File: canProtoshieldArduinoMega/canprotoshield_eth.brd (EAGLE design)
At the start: 101.3 x 80.6 mm, 54 parts, among them CN1 1X4-3.5MM, CN12 1X4-3.5MM, CN13 1X4-3.5MM, CN14 1X4-3.5MM, CN15 1X4-3.5MM, CN16 1X4-3.5MM, CN17 1X4-3.5MM, CN18 1X4-3.5MM, CN19 1X4-3.5MM, CN2 1X4-3.5MM, CN20 1X4-3.5MM, CN21 1X4-3.5MM, CN22 1X4-3.5MM, CN23 1X4-3.5MM, CN24 1X4-3.5MM, CN25 1X4-3.5MM, CN27 1X4-3.5MM, CN28 1X4-3.5MM, CN29 1X4-3.5MM, CN3 1X4-3.5MM, CN33 1X4-3.5MM, CN4 1X4-3.5MM, CN5 1X4-3.5MM, CN6 1X4-3.5MM, Q1 16mhz, U2 MCP2551, U3 ARDUINO-MEGAFULL

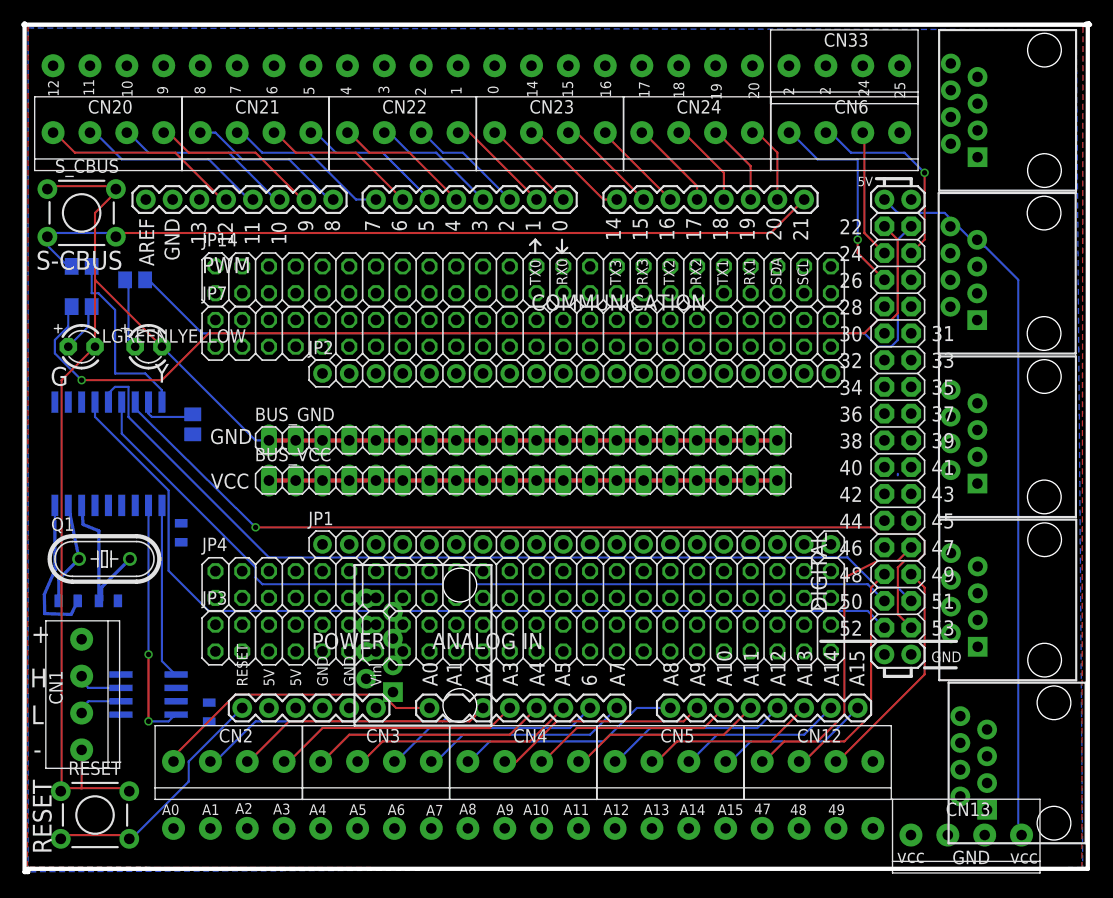
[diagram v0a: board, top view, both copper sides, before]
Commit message: Board with ethernet connectors.
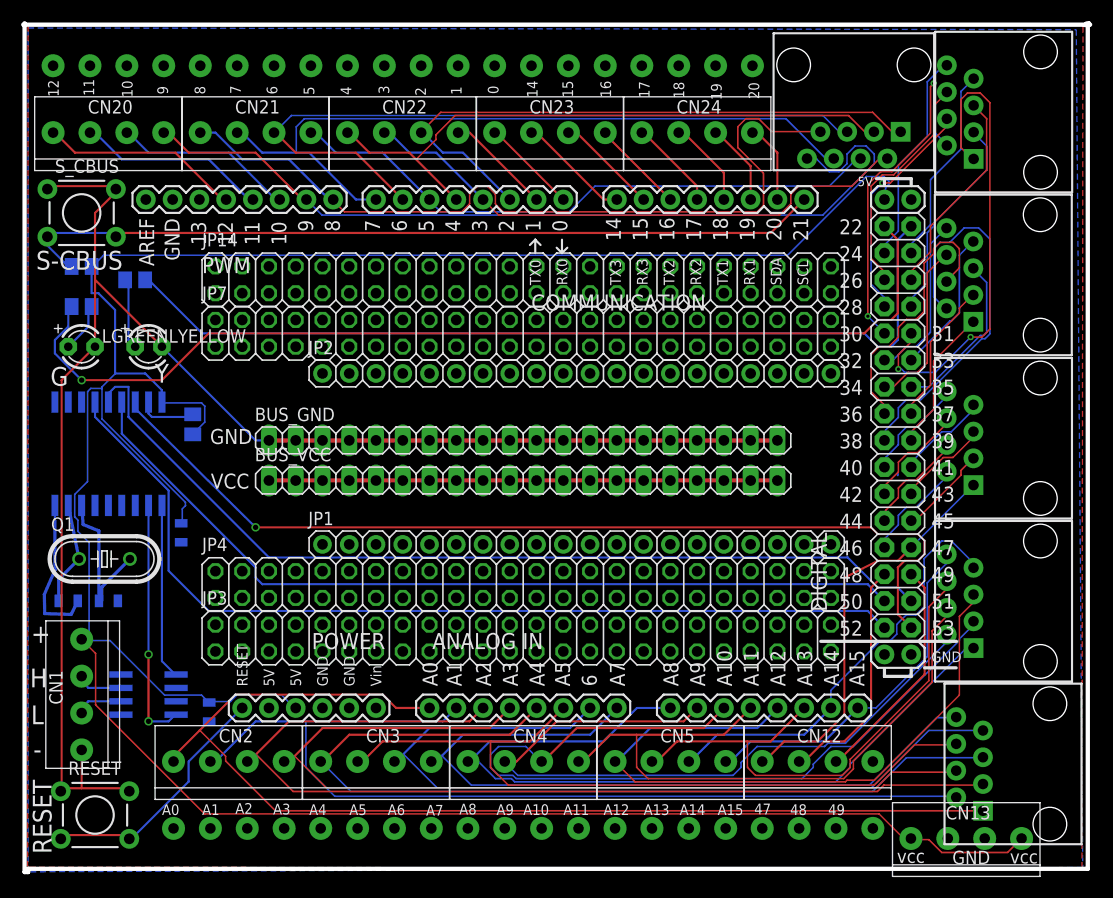
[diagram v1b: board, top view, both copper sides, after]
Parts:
- removed CN33, CN6: 1X4-3.5MM, Arduino_merg:1X04-3.5MM
- moved ANALOG 57.1 mm to (97.0, 9.93)
- moved PWM 18.6 mm to (78.4, 76.3), turned to 180 degrees
- moved ANALOG1 15.4 mm to (96.1, 25.4)
- moved DIGITAL2 15.4 mm to (96.1, 56.3)
- moved DIGITAL3 15.4 mm to (96.1, 40.8)
- moved DIGITAL1 15.3 mm to (96.1, 71.8)
- moved CN13 0.33 mm to (89.0, 2.85)
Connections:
- removed net N$53: CN6.4
- net 24: no longer CN6.3
- net 25: no longer CN6.2
- net 26: no longer CN6.1
- net GND: now also U3.GND@4
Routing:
- net VCC: track 86.3 -> 276.1 mm
- net A0: track 28.4 -> 106.2 mm
- net A2: track 24.5 -> 96.3 mm
- net A1: track 25.4 -> 92.8 mm
- net 9: track 16.2 -> 82.4 mm
- net A3: track 23.5 -> 89.5 mm
- net A4: track 22.6 -> 88.0 mm
- net 8: track 15.2 -> 77.1 mm
- net A10: track 19.4 -> 79.3 mm
- net A6: track 20.7 -> 79.3 mm
- net 6: track 14.9 -> 70.6 mm
- net 7: track 15.8 -> 71.2 mm
- net A8: track 21.3 -> 75.8 mm
- net A7: track 19.7 -> 72.4 mm
- net A5: track 21.6 -> 70.7 mm
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
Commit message: Last version with correction.
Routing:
- net GND: track 114.2 -> 114.8 mm
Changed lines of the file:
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@@
 <description language="de">&lt;b&gt;EAGLE Design Rules&lt;/b&gt;
 &lt;p&gt;
-Die Standard-Design-Rules sind so gewählt, dass sie für
+Die Standard-Design-Rules sind so gewÃ¤hlt, dass sie fÃ¼r
 die meisten Anwendungen passen. Sollte ihre Platine
 besondere Anforderungen haben, treffen Sie die erforderlichen
@@
 <autorouter>
 <pass name="Default">
-<param name="RoutingGrid" value="50mil"/>
+<param name="RoutingGrid" value="6.25mil"/>
 <param name="AutoGrid" value="1"/>
 <param name="Efforts" value="1"/>
 <param name="TopRouterVariant" value="1"/>
 <param name="tpViaShape" value="round"/>
-<param name="PrefDir.1" value="a"/>
+<param name="PrefDir.1" value="*"/>
 <param name="PrefDir.2" value="0"/>
 <param name="PrefDir.3" value="0"/>
@@
 <param name="PrefDir.14" value="0"/>
 <param name="PrefDir.15" value="0"/>
-<param name="PrefDir.16" value="a"/>
+<param name="PrefDir.16" value="*"/>
 <param name="cfVia" value="8"/>
 <param name="cfNonPref" value="5"/>
@@
 <wire x1="14.6304" y1="30.9372" x2="14.526134375" y2="30.96958125" width="0.1524" layer="16"/>
 <wire x1="14.6304" y1="30.9372" x2="14.526115625" y2="30.9372" width="0.1524" layer="16"/>
-<wire x1="8.52" y1="25.4" x2="4.71" y2="25.4" width="0" layer="19" extent="16-16"/>
-<wire x1="14.526134375" y1="30.96958125" x2="8.52" y2="25.4" width="0" layer="19" extent="16-16"/>
-<wire x1="27.94" y1="15.24" x2="17.186240625" y2="13.952403125" width="0" layer="19" extent="16-16"/>
-<wire x1="83.82" y1="20.32" x2="87.294525" y2="2.85115625" width="0" layer="19" extent="1-1"/>
+<wire x1="90.805" y1="3.175" x2="90.794525" y2="2.85115625" width="0.1524" layer="1"/>
+<wire x1="90.805" y1="3.175" x2="90.747703125" y2="2.89795625" width="0.1524" layer="1"/>
 </signal>
 <signal name="VCC">
